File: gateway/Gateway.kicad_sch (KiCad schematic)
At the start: 0 parts

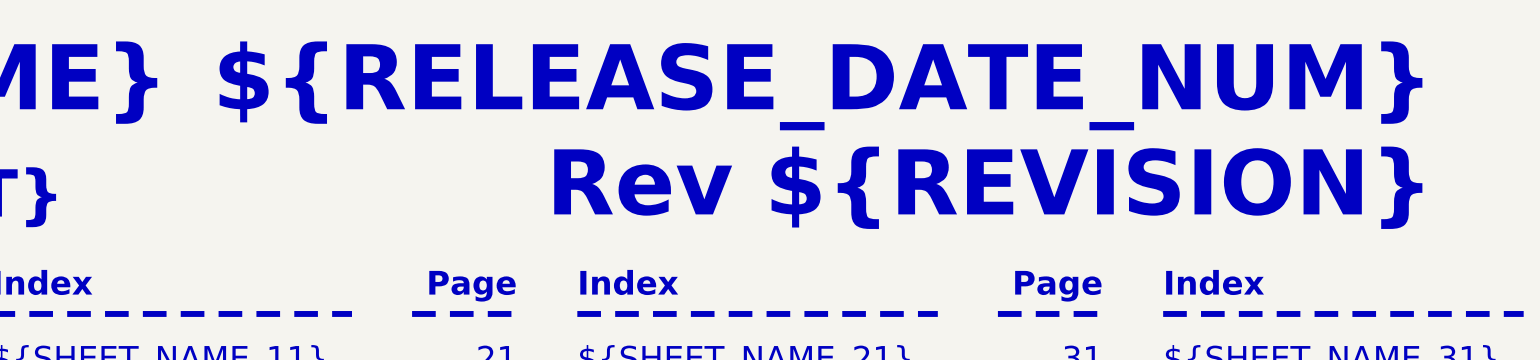
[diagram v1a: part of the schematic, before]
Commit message: Working on first version
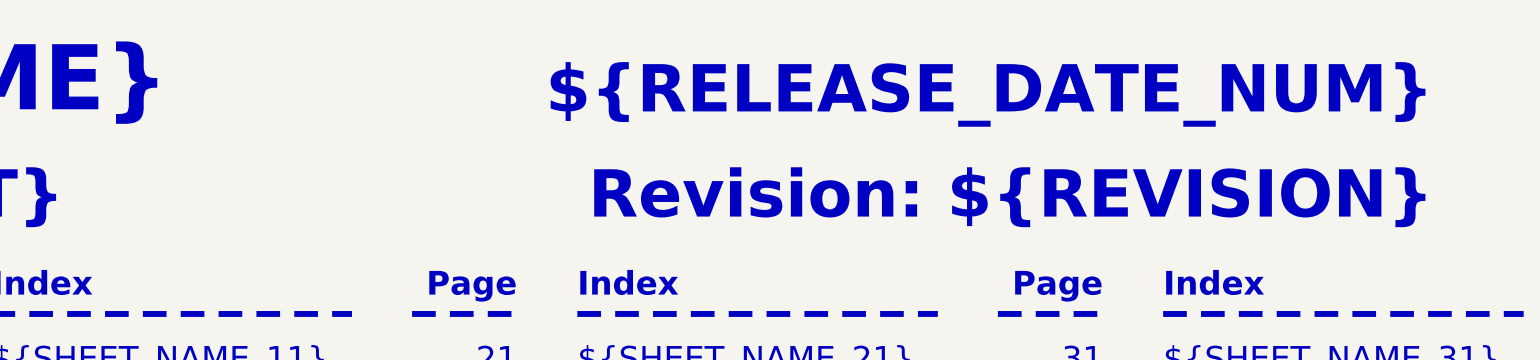
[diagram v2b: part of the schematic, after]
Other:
- note added: "Revision: ${REVISION}"
- note removed: "Rev ${REVISION}"
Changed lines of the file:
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@@
 			(font
 				(face "Times New Roman")
-				(size 11 11)
+				(size 8 8)
 				(thickness 1)
 				(bold yes)
@@
 		)
 	)
-	(text "Rev ${REVISION}"
+	(text "Revision: ${REVISION}"
 		(exclude_from_sim no)
 		(at 394.97 59.69 0)
@@
 			(font
 				(face "Times New Roman")
-				(size 11 11)
+				(size 8 8)
 				(thickness 1)
 				(bold yes)
